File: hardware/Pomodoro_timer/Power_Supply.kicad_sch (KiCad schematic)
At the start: 17 parts, among them J1 USB_C_Receptacle_USB2.0_16P, Q1 FS8205A, U1 TP4056-42-ESOP8, U2 DW01A, U3 AP2127K-3.3

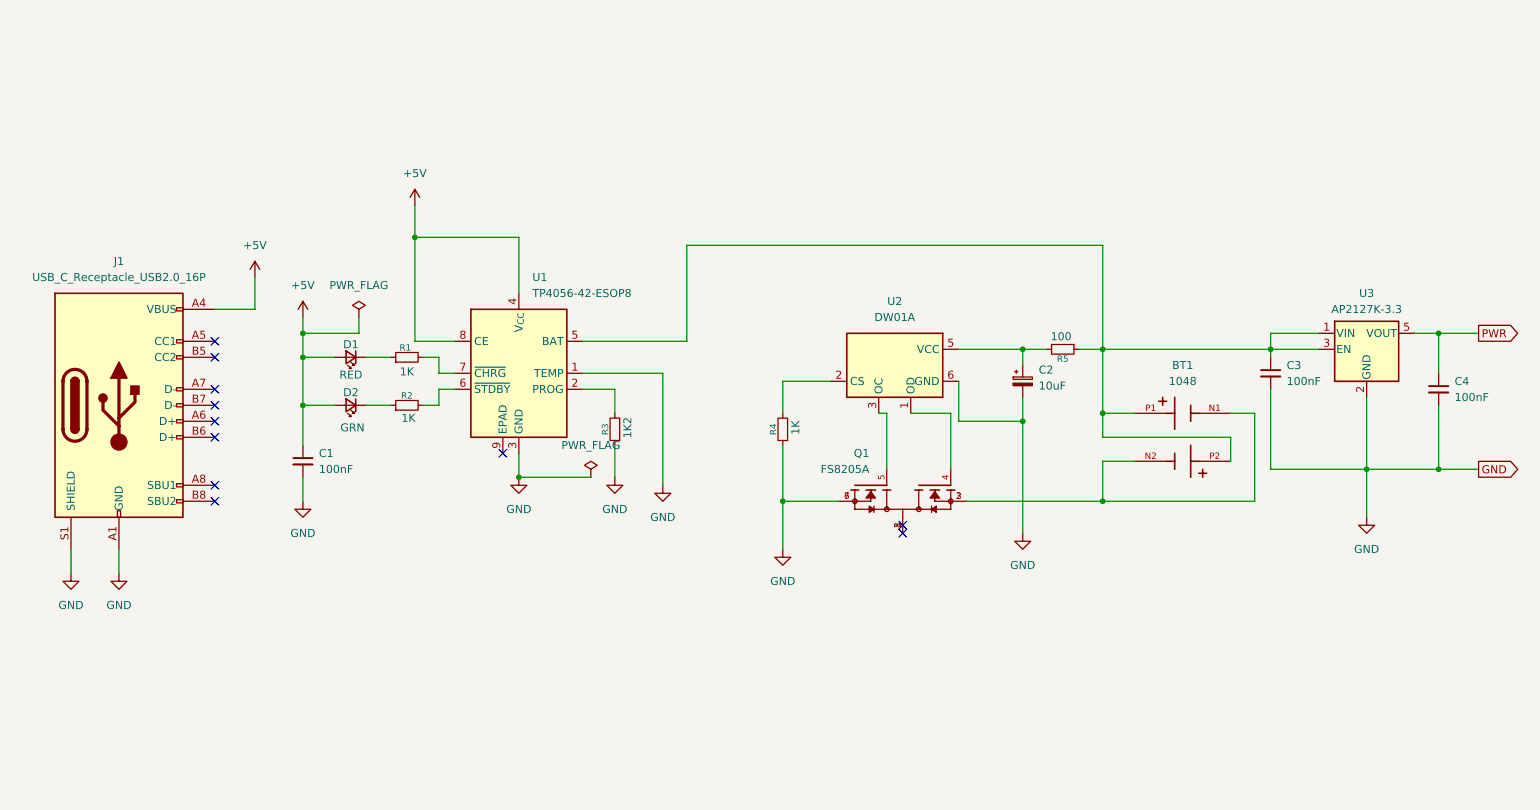
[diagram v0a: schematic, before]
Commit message: PCB Ver.A : The Schematic completed the next part for PCB can be started.
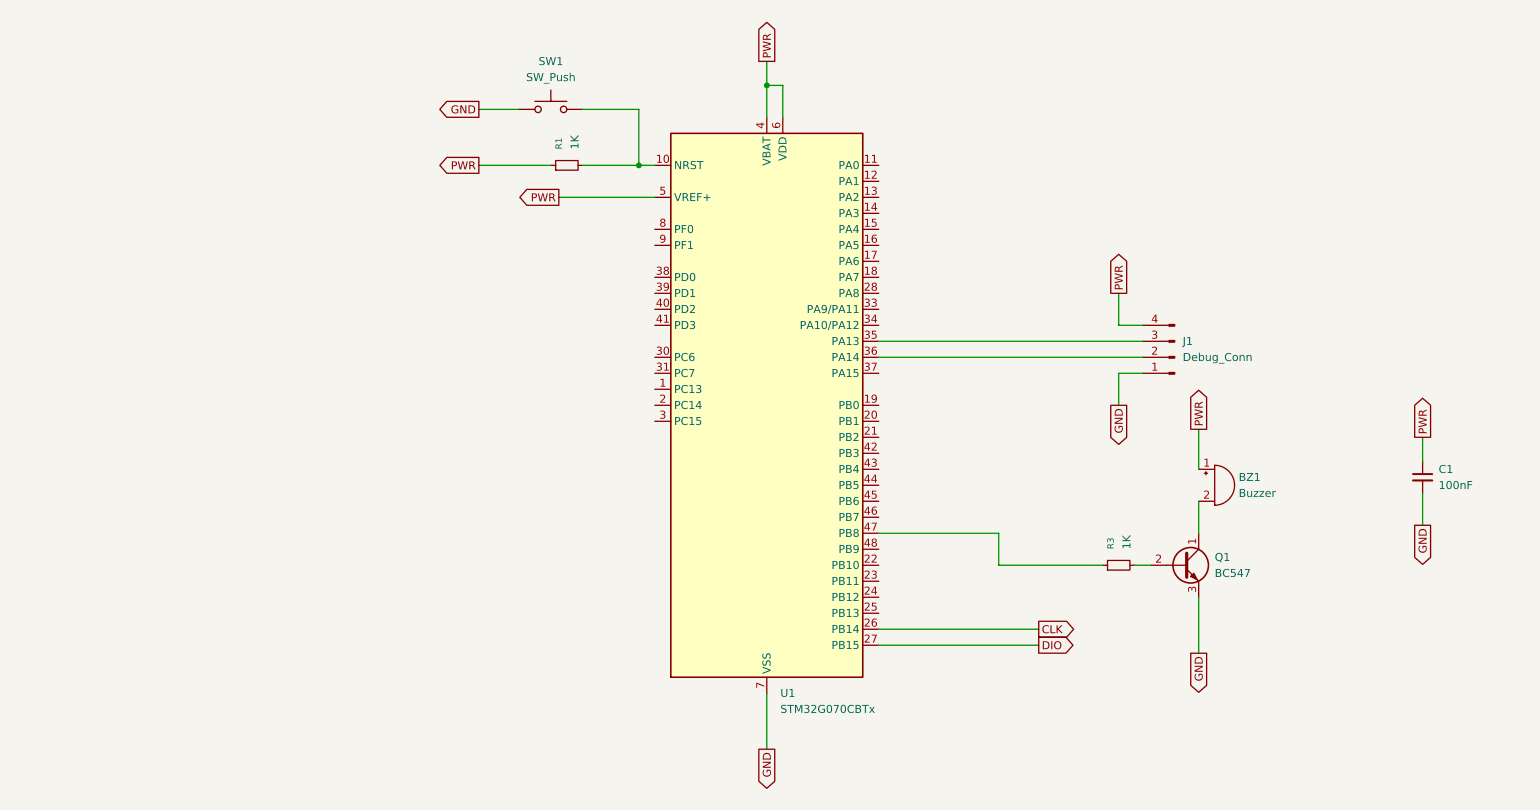
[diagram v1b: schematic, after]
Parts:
- removed BT1: 1048, 1048:BAT_1048, symbol 1048:1048
- removed C2: 10uF, symbol Device:C_Polarized_Small
- removed C3, C4: 100nF, symbol Device:C_Small
- removed D1: RED, symbol Device:LED_Small
- removed D2: GRN, symbol Device:LED_Small
- removed J1: USB_C_Receptacle_USB2.0_16P, symbol Connector:USB_C_Receptacle_USB2.0_16P
- removed Q1: FS8205A, FS8205A:SOP65P640X120-8N, symbol FS8205A:FS8205A
- removed R2, R4: 1K, symbol Device:R_Small
- removed R5: 100, symbol Device:R_Small
- removed U1: TP4056-42-ESOP8, Package_SO:SOIC-8-1EP_3.9x4.9mm_P1.27mm_EP2.41x3.3mm_ThermalVias, symbol Battery_Management:TP4056-42-ESOP8
- removed U2: DW01A, Package_TO_SOT_SMD:SOT-23-6, symbol Battery_Management:DW01A
- removed U3: AP2127K-3.3, Package_TO_SOT_SMD:SOT-223-3_TabPin2, symbol Regulator_Linear:AP2127K-3.3
- added BZ1: Buzzer, symbol Device:Buzzer
- added J1: Debug_Conn, symbol Connector:Conn_01x04_Pin
- added Q1: BC547, Package_TO_SOT_THT:TO-92, symbol Transistor_BJT:BC547
- added SW1: SW_Push, symbol Switch:SW_Push
- added U1: STM32G070CBTx, Package_QFP:LQFP-48_7x7mm_P0.5mm, symbol MCU_ST_STM32G0:STM32G070CBTx
- R3: value 1K2 -> 1K
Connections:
- net +5V is gone; now on net PWR: C1.1
- net GND: now also J1.1 (Pin_1), Q1.3 (E), SW1.1, U1.7 (VSS); no longer R3.1
- net PWR: now also R1.1, BZ1.1 (+), J1.4 (Pin_4), U1.4 (VBAT), U1.5 (VREF+), U1.6 (VDD)
- net at R3.2: now also Q1.2 (B)
- net at R1.2: now also SW1.2, U1.10 (NRST)
- new net: R3.1, U1.47 (PB8)
- new net: J1.2 (Pin_2), U1.36 (PA14)
- new net: J1.3 (Pin_3), U1.35 (PA13)
- new net: BZ1.2 (-), Q1.1 (C)
- new net CLK: U1.26 (PB14)
- new net DIO: U1.27 (PB15)
- no-connect marks 11 -> 0
